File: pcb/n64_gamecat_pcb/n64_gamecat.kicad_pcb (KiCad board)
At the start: 2 copper layers, 117.5 x 162.5 mm, 4 parts

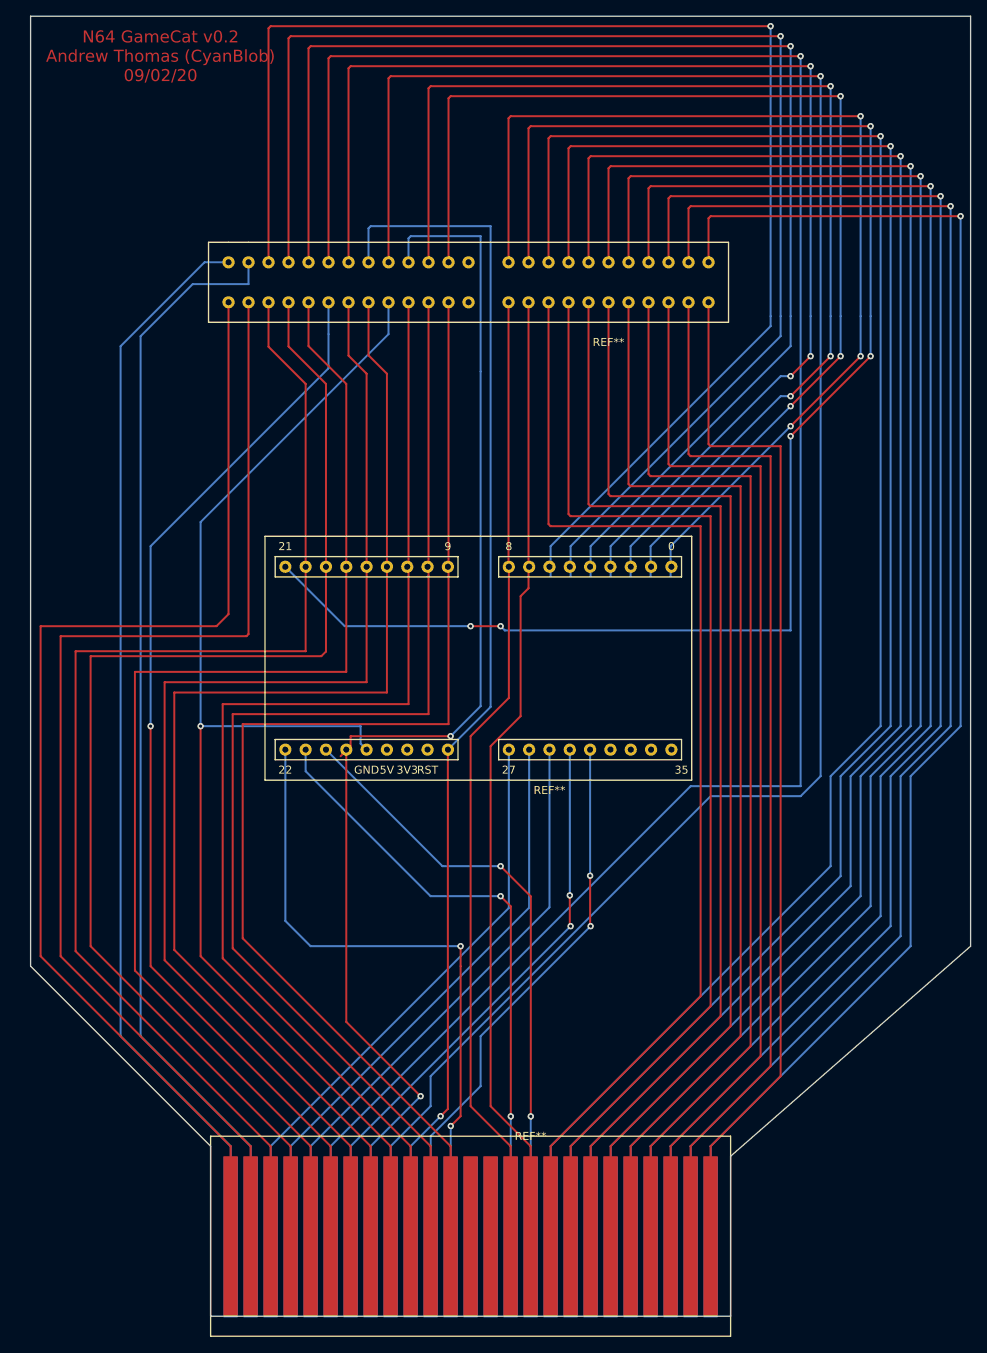
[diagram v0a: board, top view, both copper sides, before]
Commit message: Add rev 3 PCB
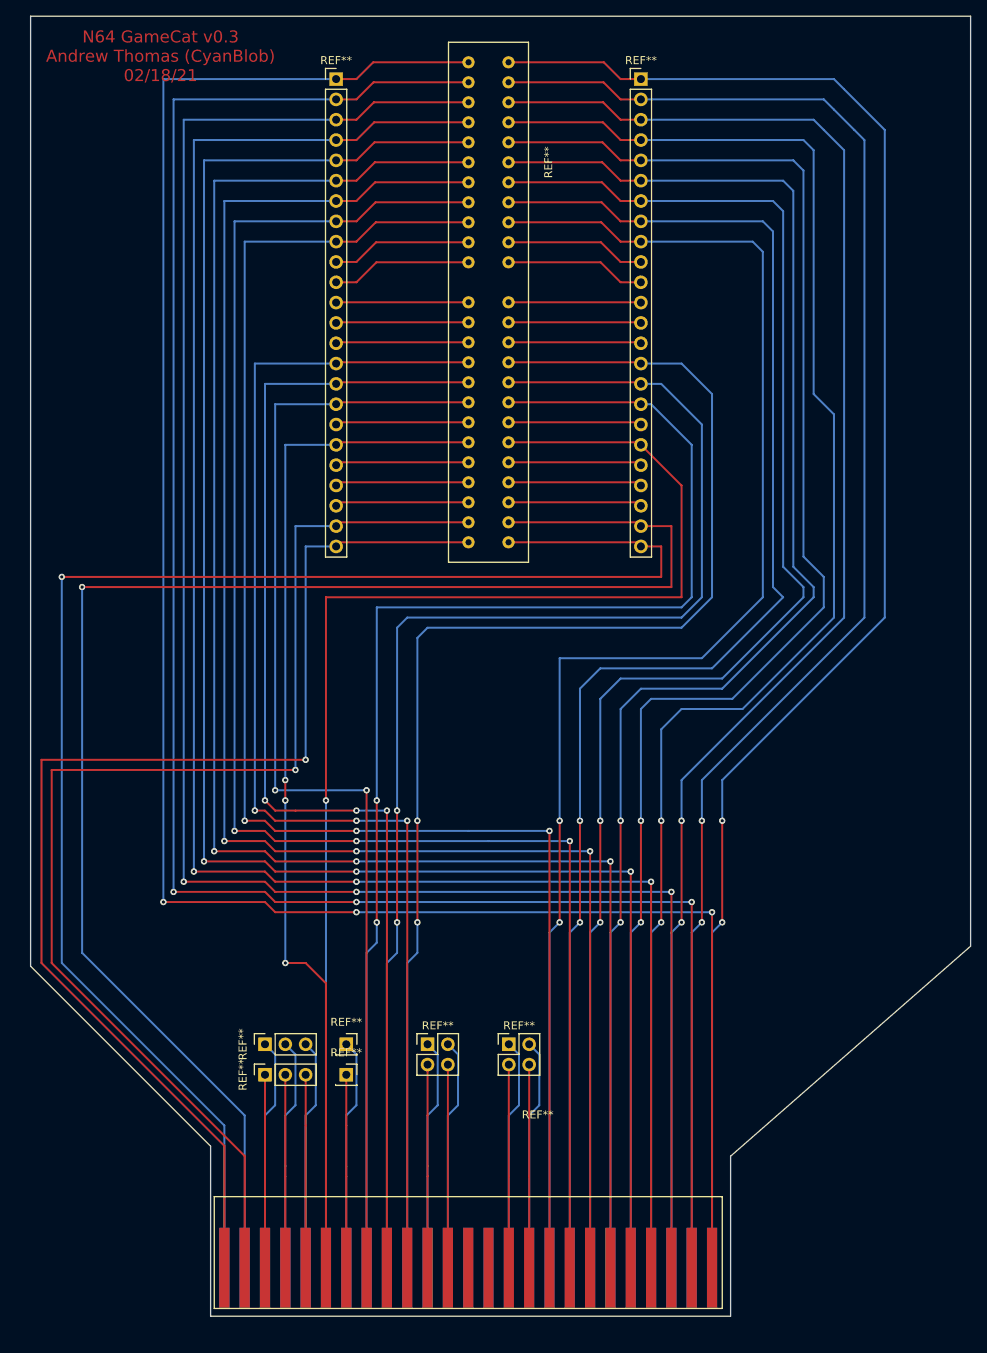
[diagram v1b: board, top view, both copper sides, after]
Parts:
- removed the REF** at (135.9, 109.2)
- added REF**: PinHeader_2x02_P2.54mm_Vertical, Connector_PinHeader_2.54mm:PinHeader_2x02_P2.54mm_Vertical, F.Cu at (144.8, 143.5)
- added REF**: PinHeader_2x02_P2.54mm_Vertical, Connector_PinHeader_2.54mm:PinHeader_2x02_P2.54mm_Vertical, F.Cu at (134.6, 143.5)
- added REF**: PinSocket_1x03_P2.54mm_Vertical, Connector_PinSocket_2.54mm:PinSocket_1x03_P2.54mm_Vertical, F.Cu at (114.3, 143.5)
- added REF**: PinSocket_1x03_P2.54mm_Vertical, Connector_PinSocket_2.54mm:PinSocket_1x03_P2.54mm_Vertical, F.Cu at (114.3, 147.3)
- added REF**: PinSocket_1x01_P2.54mm_Vertical, Connector_PinSocket_2.54mm:PinSocket_1x01_P2.54mm_Vertical, F.Cu at (124.5, 147.3)
- added REF**: PinSocket_1x01_P2.54mm_Vertical, Connector_PinSocket_2.54mm:PinSocket_1x01_P2.54mm_Vertical, F.Cu at (124.5, 143.5)
- added REF**: PinHeader_1x24_P2.54mm_Vertical, Connector_PinHeader_2.54mm:PinHeader_1x24_P2.54mm_Vertical, F.Cu at (161.3, 22.9)
- added REF**: PinHeader_1x24_P2.54mm_Vertical, Connector_PinHeader_2.54mm:PinHeader_1x24_P2.54mm_Vertical, F.Cu at (123.2, 22.9)
- moved REF** 10.5 mm to (135.9, 195.6)
- moved REF** 2.82 mm to (135.9, 147.3)
- turned REF** to 90 degrees
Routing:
- net (no net): track 8006.9 -> 6430.2 mm, vias 46 -> 67
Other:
- board text added: "N64 GameCat v0.3 Andrew Thomas (CyanBlob) 02/18/21"
- board text removed: "N64 GameCat v0.2 Andrew Thomas (CyanBlob) 09/02/20"
